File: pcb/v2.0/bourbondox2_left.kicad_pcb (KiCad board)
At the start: 2 copper layers, 181 x 154.8 mm, 63 parts, among them J1 MJ-4PP-9, SW1 SW_Push, U1 ProMicro

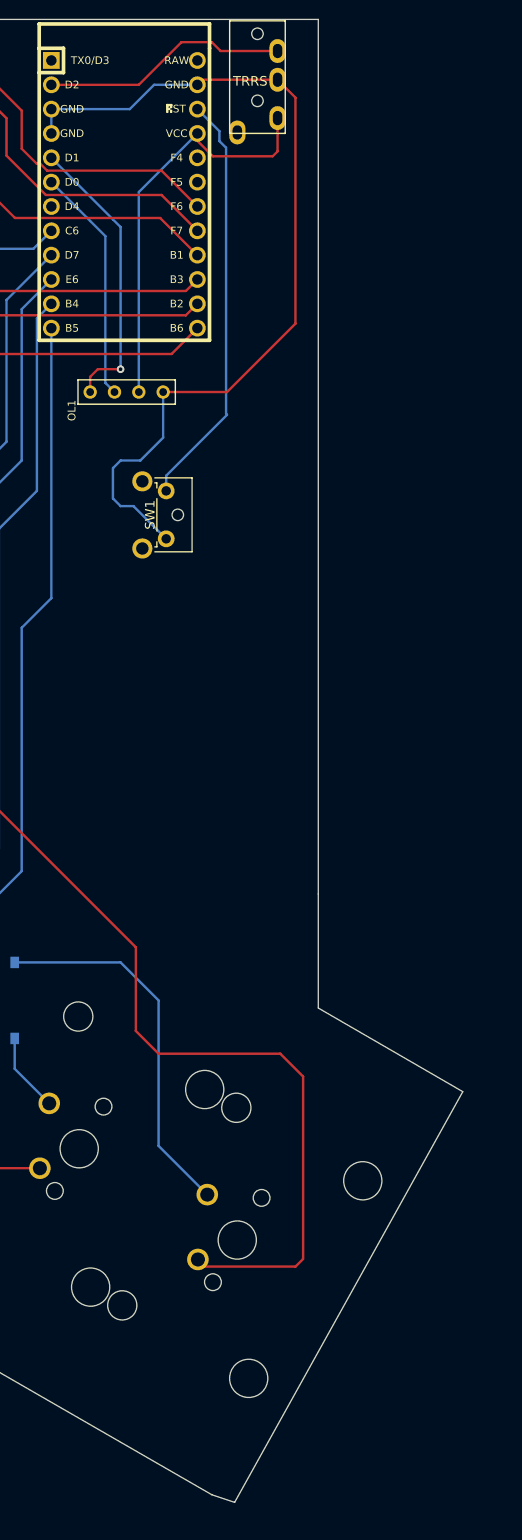
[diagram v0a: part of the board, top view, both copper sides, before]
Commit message: Cleaning files off Asus ZenBook
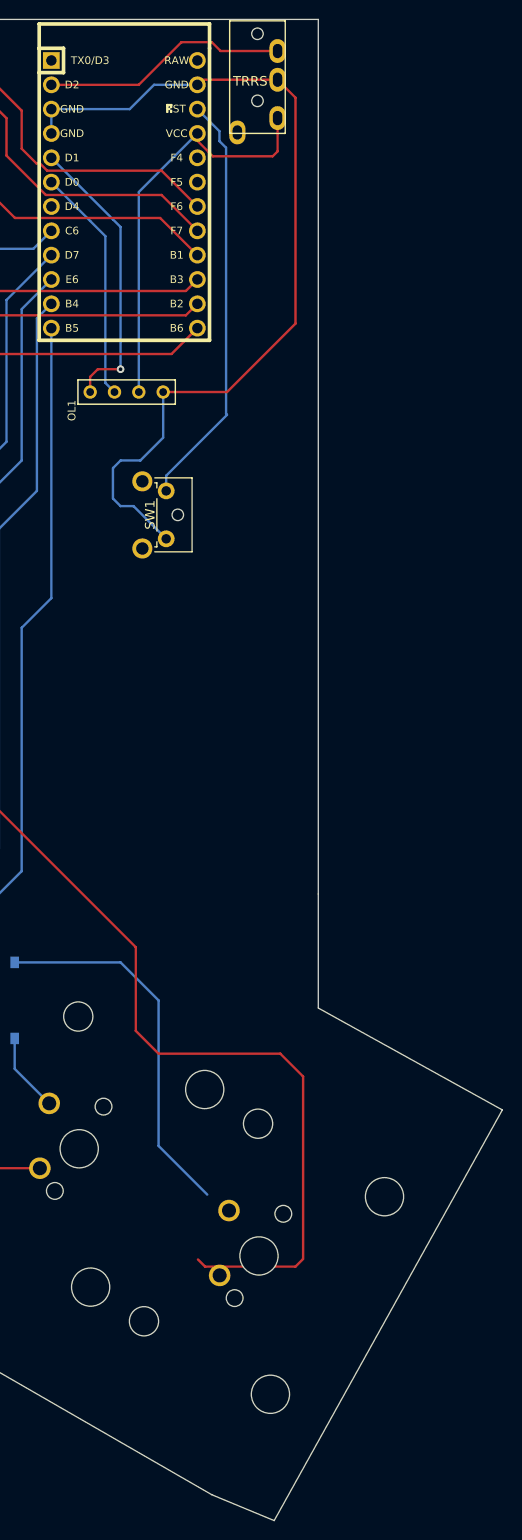
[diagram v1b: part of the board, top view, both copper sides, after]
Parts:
- moved MX45 2.81 mm to (243.8, 147.3)
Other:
- board size 181 x 154.8 mm -> 185.1 x 156.7 mm
- net class Default removed
